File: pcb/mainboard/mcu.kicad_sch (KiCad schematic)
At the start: 41 parts, among them J5 2x6_1.27_HDR, J7 MICRO_SD(TFC-WPAPR-08), SW1 SW, SW2 SW, SW3 SW, U14 W25Q32JV, U3 STM32H750VBTx, Y1 24MHz, Y2 32.768K

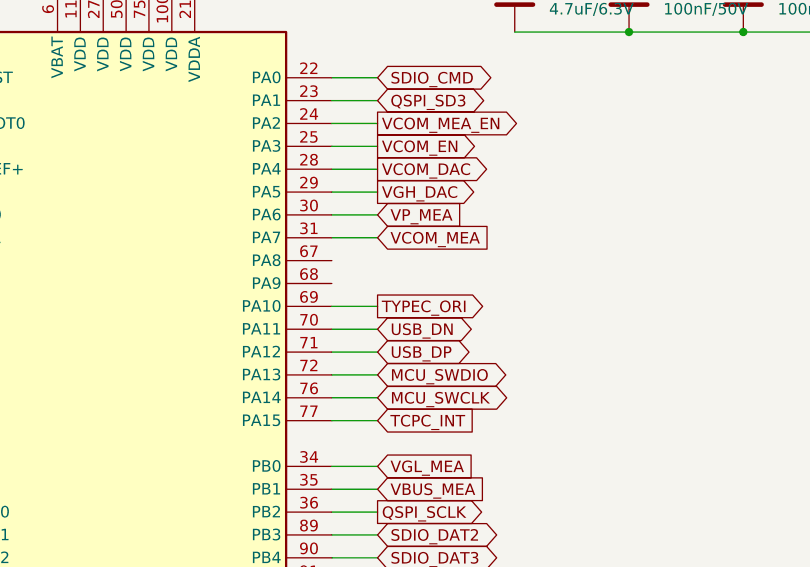
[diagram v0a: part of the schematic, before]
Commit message: PCB r1p3
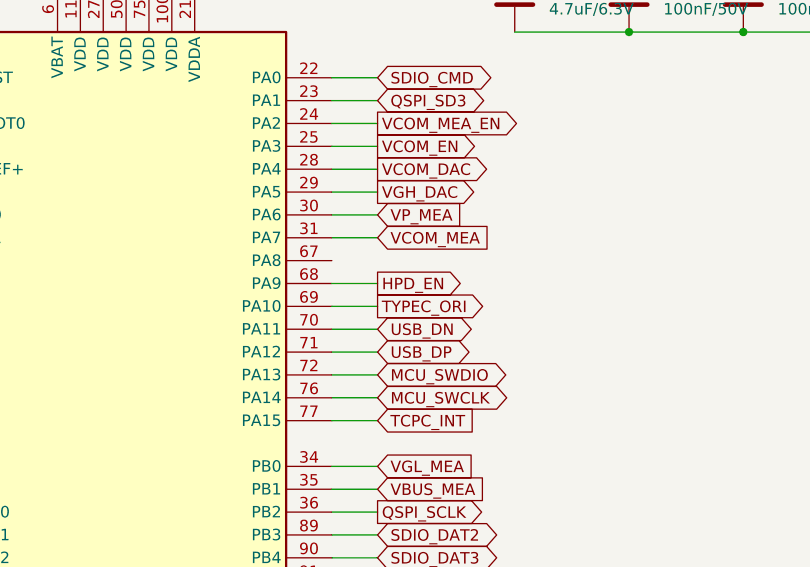
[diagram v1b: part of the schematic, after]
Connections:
- net HPD_EN: now reaches U3.68 (PA9)
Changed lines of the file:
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@@
+	(wire
+		(pts
+			(xy 91.44 60.96) (xy 96.52 60.96)
+		)
+		(stroke
+			(width 0)
+			(type default)
+		)
+	)
 	(wire
 		(pts
@@
 	(label "G_LED"
 		(at 33.02 60.96 0)
-		(fields_autoplaced yes)
 		(effects
 			(font
@@
 	(label "G_LED"
 		(at 106.68 170.18 0)
-		(fields_autoplaced yes)
 		(effects
 			(font
@@
 	(label "OSC_IN"
 		(at 33.02 53.34 0)
-		(fields_autoplaced yes)
 		(effects
 			(font
@@
 	(label "OSC_IN"
 		(at 200.66 58.42 180)
-		(fields_autoplaced yes)
 		(effects
 			(font
@@
 	(label "OSC_OUT"
 		(at 200.66 71.12 180)
-		(fields_autoplaced yes)
 		(effects
 			(font
@@
 	(label "OSC32_OUT"
 		(at 104.14 162.56 180)
-		(fields_autoplaced yes)
 		(effects
 			(font
@@
 	(label "OSC32_IN"
 		(at 200.66 88.9 180)
-		(fields_autoplaced yes)
 		(effects
 			(font
@@
 	(label "OSC32_IN"
 		(at 104.14 160.02 180)
-		(fields_autoplaced yes)
 		(effects
 			(font
@@
 	(label "OSC32_OUT"
 		(at 200.66 101.6 180)
-		(fields_autoplaced yes)
 		(effects
 			(font
@@
 	(label "R_LED"
 		(at 33.02 63.5 0)
-		(fields_autoplaced yes)
 		(effects
 			(font
@@
 	(label "R_LED"
 		(at 106.68 175.26 0)
-		(fields_autoplaced yes)
 		(effects
 			(font
@@
 	(label "OSC_OUT"
 		(at 33.02 55.88 0)
-		(fields_autoplaced yes)
 		(effects
 			(font
@@
 				(hide yes)
 			)
+		)
+	)
+	(global_label "HPD_EN"
+		(shape output)
+		(at 96.52 60.96 0)
+		(fields_autoplaced yes)
+		(effects
+			(font
+				(size 1.27 1.27)
+			)
+			(justify left)
+		)
+		(property "Intersheetrefs" "${INTERSHEET_REFS}"
+			(at 106.8228 60.96 0)
+			(effects
+				(font
+					(size 1.27 1.27)
+				)
+				(justify left)
+				(hide yes)
+			)

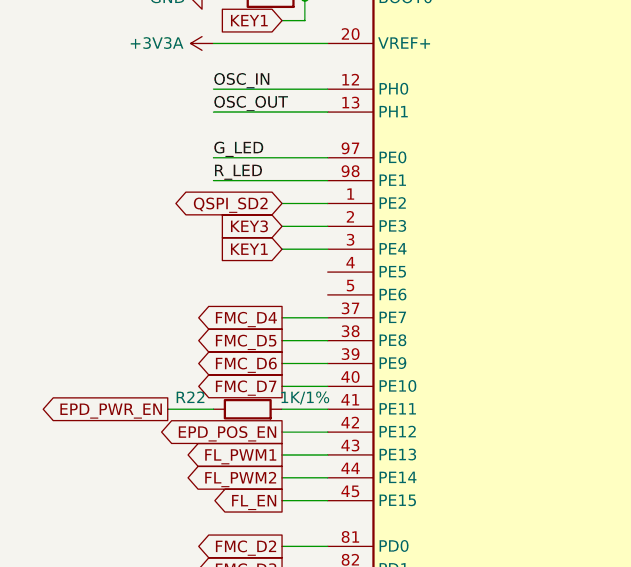
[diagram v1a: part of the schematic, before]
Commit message: Sync local PCB changes
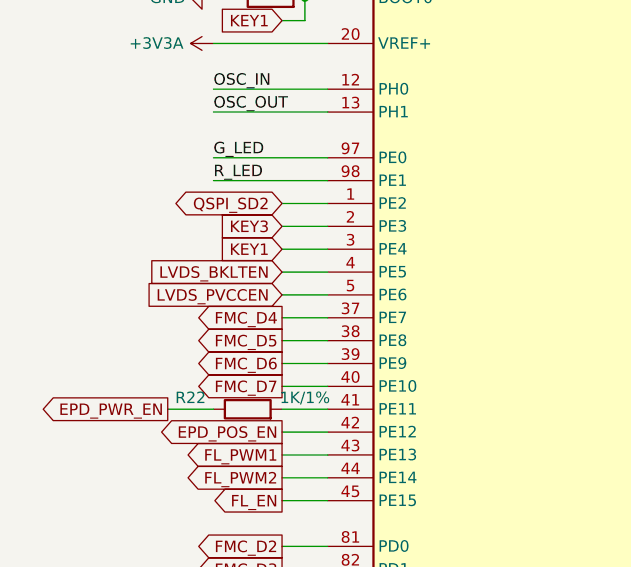
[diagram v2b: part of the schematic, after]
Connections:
- net LVDS_BKLTEN: now reaches U3.4 (PE5)
- net LVDS_PVCCEN: now reaches U3.5 (PE6)
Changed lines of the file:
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@@
+	(wire
+		(pts
+			(xy 45.72 73.66) (xy 40.64 73.66)
+		)
+		(stroke
+			(width 0)
+			(type default)
+		)
+	)
 	(wire
 		(pts
@@
 		(pts
 			(xy 203.2 33.02) (xy 215.9 33.02)
+		)
+		(stroke
+			(width 0)
+			(type default)
+		)
+	)
+	(wire
+		(pts
+			(xy 45.72 76.2) (xy 40.64 76.2)
 		)
 		(stroke
@@
 		)
 	)
+	(global_label "LVDS_BKLTEN"
+		(shape input)
+		(at 40.64 73.66 180)
+		(fields_autoplaced yes)
+		(effects
+			(font
+				(size 1.27 1.27)
+			)
+			(justify right)
+		)
+		(property "Intersheetrefs" "${INTERSHEET_REFS}"
+			(at 25.0758 73.66 0)
+			(effects
+				(font
+					(size 1.27 1.27)
+				)
+				(justify right)
+				(hide yes)
+			)
+		)
+	)
 	(global_label "SDIO_DAT1"
 		(shape bidirectional)
@@
 			(effects
 				(font
+					(size 1.27 1.27)
+				)
+				(justify right)
+				(hide yes)
+			)
+		)
+	)
+	(global_label "LVDS_PVCCEN"
+		(shape input)
+		(at 40.64 76.2 180)
+		(fields_autoplaced yes)
+		(effects
+			(font
+				(size 1.27 1.27)
+			)
+			(justify right)
+		)
+		(property "Intersheetrefs" "${INTERSHEET_REFS}"
+			(at 24.7129 76.2 0)
+			(effects
+				(font
